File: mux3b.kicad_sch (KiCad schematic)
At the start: 7 parts, among them U1 4081, U10 4071, U18 4069, U27 4069, U46 4071, U48 4081, U6 4081

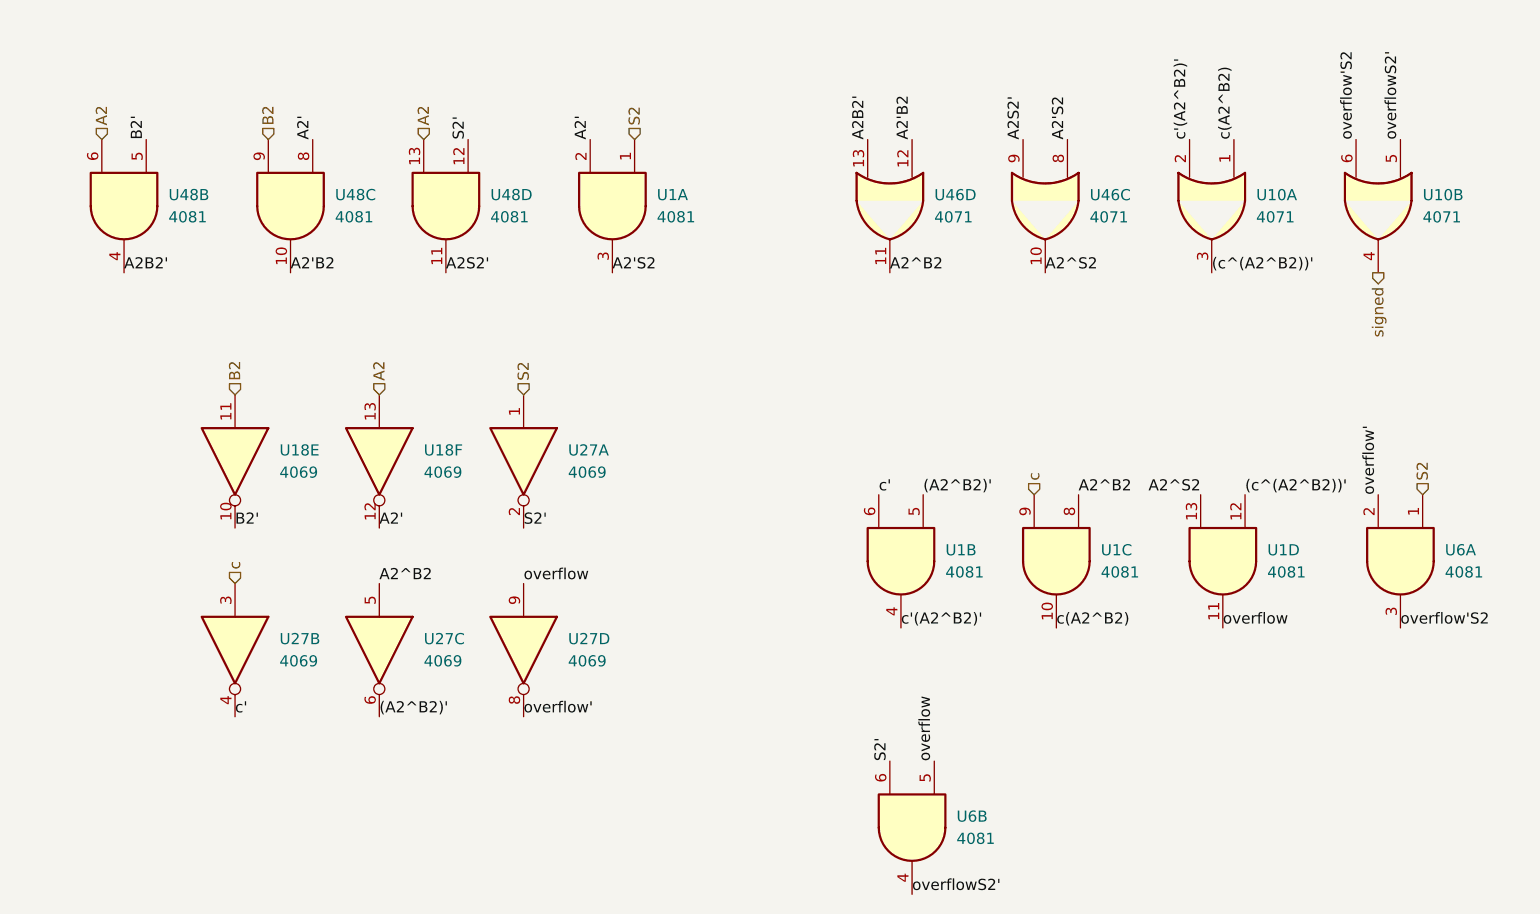
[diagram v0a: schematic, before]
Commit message: Add files via upload
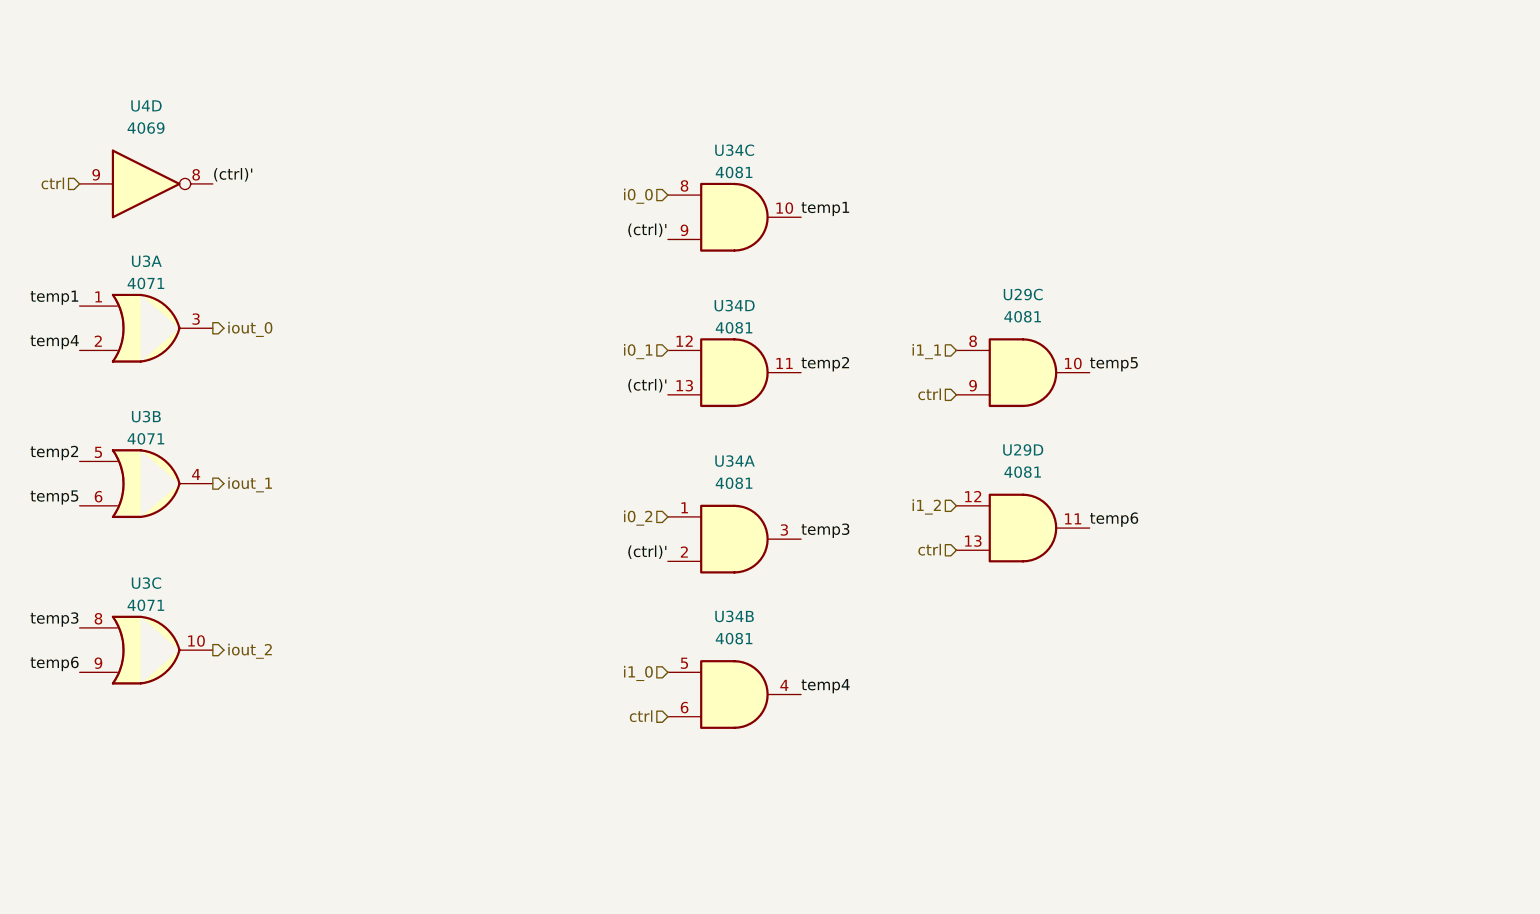
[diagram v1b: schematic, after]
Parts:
- removed U1, U48, U6: 4081, Package_DIP:CERDIP-14_W7.62mm_SideBrazed_LongPads_Socket, symbol 4xxx:4081
- removed U10, U46: 4071, Package_DIP:CERDIP-14_W7.62mm_SideBrazed_LongPads_Socket, symbol 4xxx:4071
- removed U18, U27: 4069, Package_DIP:CERDIP-14_W7.62mm_SideBrazed_LongPads_Socket, symbol 4xxx:4069
- added U29, U34: 4081, Package_DIP:CERDIP-14_W7.62mm_SideBrazed_LongPads_Socket, symbol 4xxx:4081
- added U3: 4071, Package_DIP:CERDIP-14_W7.62mm_SideBrazed_LongPads_Socket, symbol 4xxx:4071
- added U4: 4069, Package_DIP:CERDIP-14_W7.62mm_SideBrazed_LongPads_Socket, symbol 4xxx:4069
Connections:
- new net (ctrl)': U34.13, U34.2, U34.9, U4.8
- new net ctrl: U29.13, U29.9, U34.6, U4.9
- new net i0_0: U34.8
- new net i0_1: U34.12
- new net i0_2: U34.1
- new net i1_0: U34.5
- new net i1_1: U29.8
- new net i1_2: U29.12
- new net iout_0: U3.3
- new net iout_1: U3.4
- new net iout_2: U3.10
- new net temp1: U3.1, U34.10
- new net temp2: U3.5, U34.11
- new net temp3: U3.8, U34.3
- new net temp4: U3.2, U34.4
- new net temp5: U29.10, U3.6
- new net temp6: U29.11, U3.9
